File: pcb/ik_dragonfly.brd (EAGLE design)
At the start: 41.1 x 20.3 mm, 32 parts, among them IC1 FT230X, IC2 ATXMEGA32E5, J1 2X03, U1 MIC5219-3.3, U2 LM4040

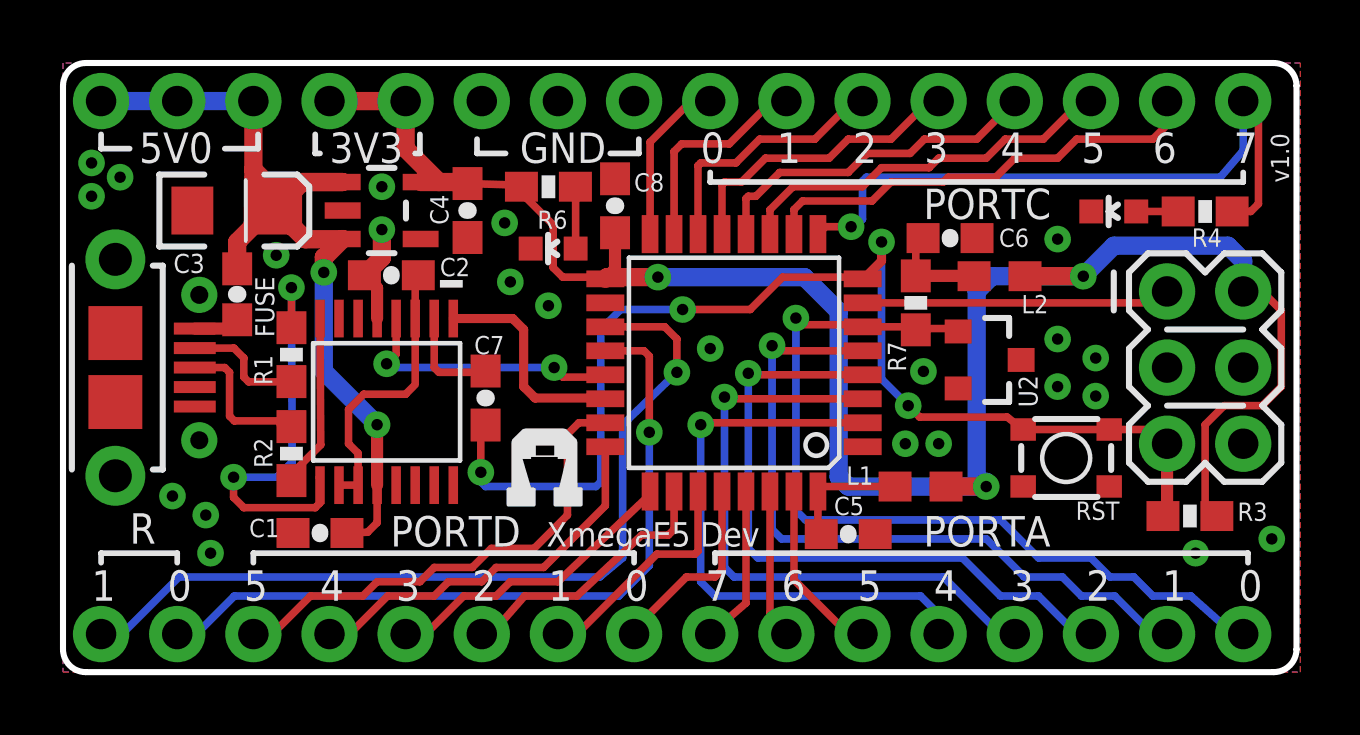
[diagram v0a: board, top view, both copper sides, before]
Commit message: updated BOM
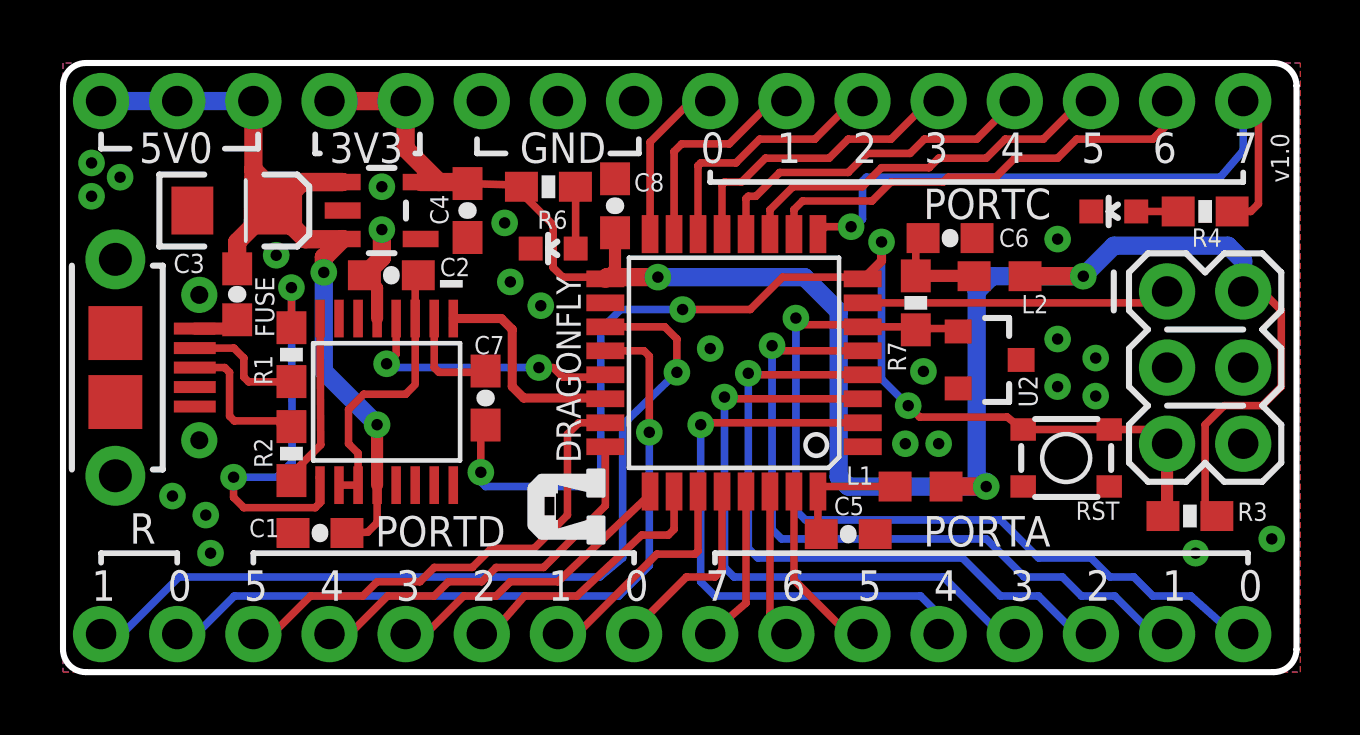
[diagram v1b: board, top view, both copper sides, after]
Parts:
- IC1: value FT230X -> ATXMEGA32E5; device Ai_IC:SSOP-16-FTDI -> Ai_IC:TQFP32-08
- IC2: value ATXMEGA32E5 -> FT230X; device Ai_IC:TQFP32-08 -> Ai_IC:SSOP-16-FTDI
- L: value (none) -> YELLOW
- L1, L2: value (none) -> 33@100MHz
- ON: value (none) -> BLUE
- R1, R2: value (none) -> 22
- R3, R6: value (none) -> 1K
- R4: value (none) -> 330
- moved IC1 11.7 mm to (22.4, 10.3)
- moved IC2 11.7 mm to (10.8, 9.02)
- moved U$3 3.66 mm to (18.2, 4.19), turned to 90 degrees
- renumbered LED1 to ON, LED2 to L
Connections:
- net !RTS: now also IC2.2; no longer IC1.2
- net 3V3: now also IC1.17; no longer IC2.17
- net 5V: now also IC2.12; no longer IC1.12
- net AVCC: now also IC1.32; no longer IC2.32
- net D+: now also IC2.8; no longer IC1.8
- net D-: now also IC2.9; no longer IC1.9
- net FT_3V3: now also IC2.10, IC2.11, IC2.3; no longer IC1.10, IC1.11, IC1.3
- net FT_RX: now also IC1.21, IC2.4; no longer IC1.4, IC2.21
- net FT_TX: now also IC1.22, IC2.1; no longer IC1.1, IC2.22
- net GND: now also IC1.1, IC1.18, IC2.13, IC2.5; no longer IC1.13, IC1.5, IC2.1, IC2.18
- net PA0: now also IC1.6; no longer IC2.6
- net PA1: now also IC1.5; no longer IC2.5
- net PA2: now also IC1.4; no longer IC2.4
- net PA3: now also IC1.3; no longer IC2.3
- net PA4: now also IC1.2; no longer IC2.2
- net PA5: now also IC1.31; no longer IC2.31
- net PA6: now also IC1.30; no longer IC2.30
- net PA7: now also IC1.29; no longer IC2.29
- net PC0: now also IC1.16; no longer IC2.16
- net PC1: now also IC1.15; no longer IC2.15
- net PC2: now also IC1.14; no longer IC2.14
- net PC3: now also IC1.13; no longer IC2.13
- net PC4: now also IC1.12; no longer IC2.12
- net PC5: now also IC1.11; no longer IC2.11
- net PC6: now also IC1.10; no longer IC2.10
- net PC7: now also IC1.9; no longer IC2.9
- net PD0: now also IC1.28; no longer IC2.28
- net PD1: now also IC1.27; no longer IC2.27
- net PD2: now also IC1.26; no longer IC2.26
- net PD3: now also IC1.25; no longer IC2.25
- net PD4: now also IC1.24; no longer IC2.24
- net PD5: now also IC1.23; no longer IC2.23
- net PDI_C: now also IC1.8; no longer IC2.8
- net PDI_D: now also IC1.7; no longer IC2.7
- net PR0: now also IC1.20; no longer IC2.20
- net PR1: now also IC1.19; no longer IC2.19
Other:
- board text added: "DRAGONFLY"
- board text removed: "XmegaE5 Dev"
